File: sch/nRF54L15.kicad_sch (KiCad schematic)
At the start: 13 parts, among them U2 nPM1300-QEXX

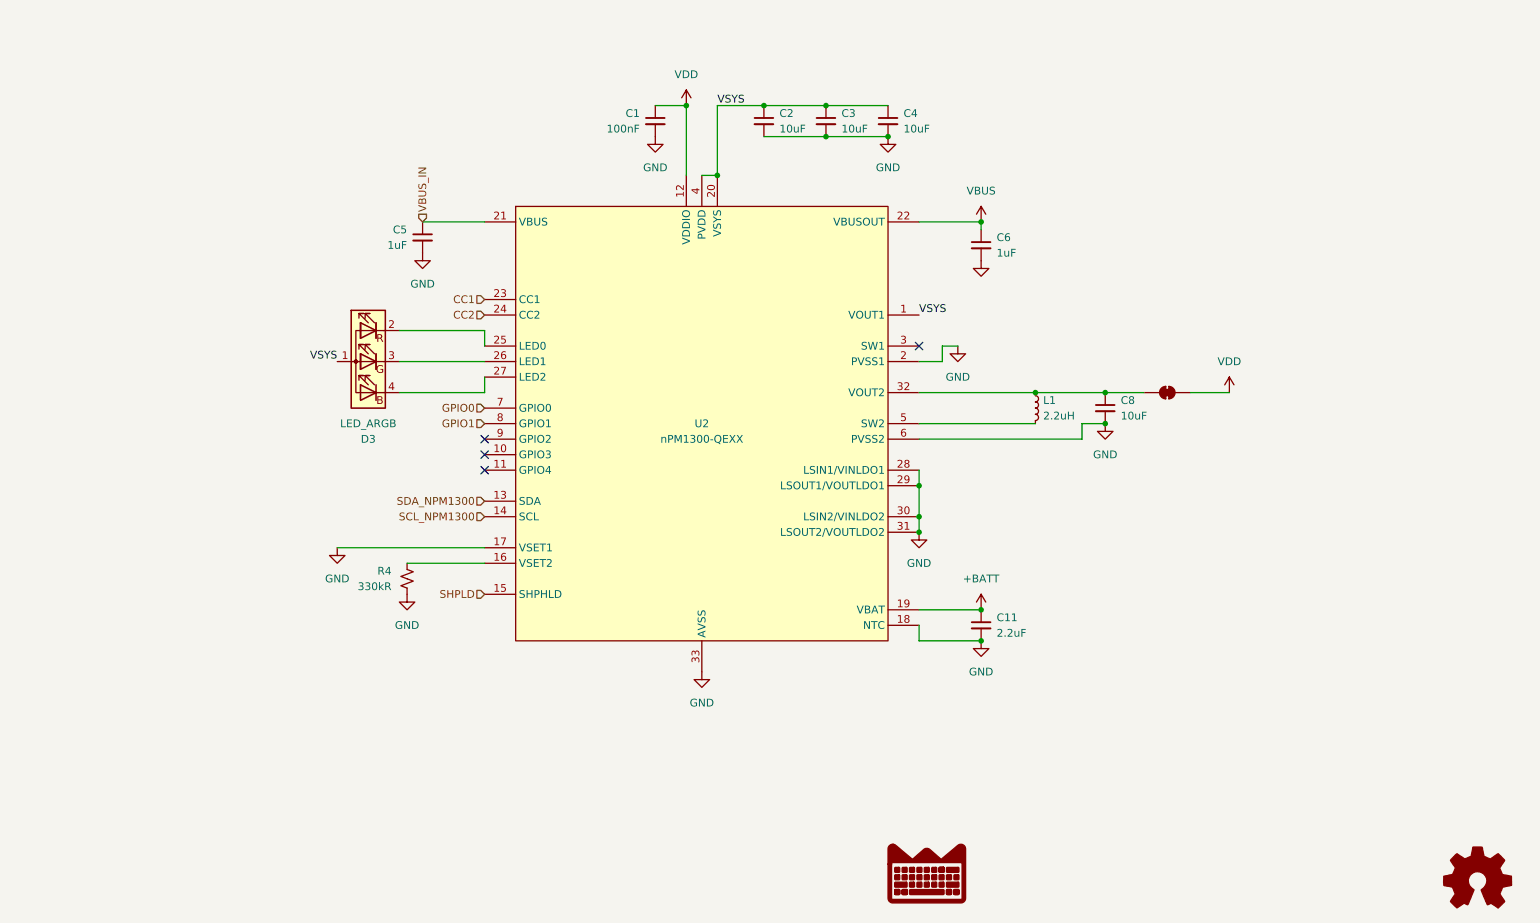
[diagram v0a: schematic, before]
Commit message: Updated 02/03/25
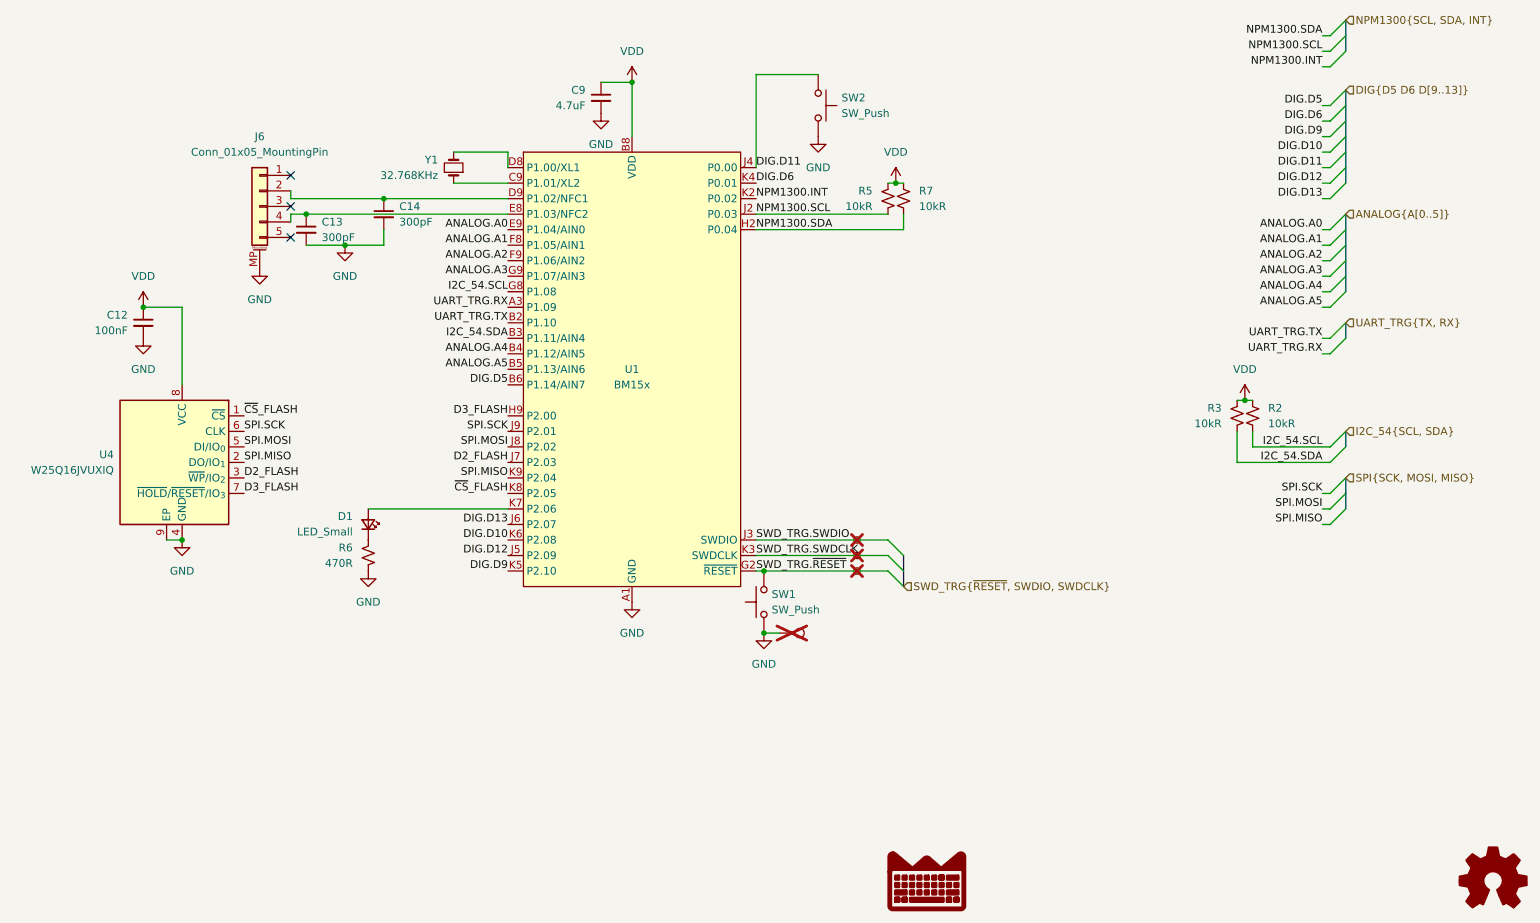
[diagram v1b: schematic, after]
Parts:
- removed C1: 100nF, Capacitor_SMD:C_0402_1005Metric, symbol Device:C_Small
- removed C11: 2.2uF, Capacitor_SMD:C_0603_1608Metric, symbol Device:C_Small
- removed C2, C3, C4, C8: 10uF, Capacitor_SMD:C_0603_1608Metric, symbol Device:C_Small
- removed C5, C6: 1uF, Capacitor_SMD:C_0603_1608Metric, symbol Device:C_Small
- removed D3: LED_ARGB, LED_SMD:LED_Wurth_150044M155260, symbol Device:LED_ARGB
- removed JP1: SolderJumper_2_Bridged, Jumper:SolderJumper-2_P1.3mm_Bridged_RoundedPad1.0x1.5mm, symbol Jumper:SolderJumper_2_Bridged
- removed L1: 2.2uH, Inductor_SMD:L_0603_1608Metric, symbol Device:L_Small
- removed R4: 330kR, Resistor_SMD:R_0402_1005Metric, symbol Device:R_Small_US
- removed U2: nPM1300-QEXX, Package_DFN_QFN:QFN-32-1EP_5x5mm_P0.5mm_EP3.6x3.6mm_ThermalVias, symbol nordic-lib-kicad-npm:nPM1300-QEXX
- added C12: 100nF, Capacitor_SMD:C_0402_1005Metric, symbol Device:C_Small
- added C13, C14: 300pF, Capacitor_SMD:C_0402_1005Metric, symbol Device:C_Small
- added C9: 4.7uF, Capacitor_SMD:C_0402_1005Metric, symbol Device:C_Small
- added D1: LED_Small, LED_SMD:LED_0603_1608Metric, symbol Device:LED_Small
- added J6: Conn_01x05_MountingPin, RoyalBlue-nRF54L15-Connector_FFC-FPC:CONN-SMD_5P-P0.50_HCTL_HC-FPC-05-09-5RLTAG, symbol Connector_Generic_MountingPin:Conn_01x05_MountingPin
- added R2, R3, R5, R7: 10kR, Resistor_SMD:R_0402_1005Metric, symbol Device:R_Small_US
- added R6: 470R, Resistor_SMD:R_0402_1005Metric, symbol Device:R_Small_US
- added SW1, SW2: SW_Push, Button_Switch_SMD:SW_Push_1P1T_NO_Vertical_Wuerth_434133025816, symbol Switch:SW_Push
- added TP1, TP2, TP3: TestPoint, TestPoint:TestPoint_Pad_D2.0mm, symbol Connector:TestPoint_Small
- added TP4: TestPoint, TestPoint:TestPoint_Pad_D2.0mm, symbol Connector:TestPoint
- added U1: BM15x, nordic-lib-kicad-nrf54-modules:BM15x-LGA-45_15.8x10mm, symbol nordic-lib-kicad-nrf54-modules:BM15x
- added U4: W25Q16JVUXIQ, Package_SON:Winbond_USON-8-1EP_3x2mm_P0.5mm_EP0.2x1.6mm, symbol Memory_Flash:W25Q32JVZP
- added Y1: 32.768KHz, Crystal:Crystal_SMD_3215-2Pin_3.2x1.5mm, symbol Device:Crystal_Small
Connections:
- net GND: now also C12.2, C13.2, C14.2, C9.2, J6.MP (MountPin), R6.2, SW1.1, SW2.2, TP4.1, U1.A1 (GND), U1.A9 (GND), U1.B1 (GND), U1.B7 (GND), U1.B9 (GND), U1.D1 (GND), U1.E1 (GND), U1.F1 (GND), U1.H8 (GND), U4.4 (GND), U4.9 (EP)
- net VDD: now also C12.1, C9.1, R2.1, R3.1, R5.1, R7.1, U1.B8 (VDD), U1.C8 (VDD), U4.8 (VCC)
- new net: D1.1 (K), R6.1
- new net: D1.2 (A), U1.K7 (P2.06)
- new net: U1.C9 (P1.01/XL2), Y1.1
- new net: U1.D8 (P1.00/XL1), Y1.2
- new net: C14.1, J6.2 (Pin_2), U1.D9 (P1.02/NFC1)
- new net: C13.1, J6.4 (Pin_4), U1.E8 (P1.03/NFC2)
- new net ANALOG.A0: U1.E9 (P1.04/AIN0)
- new net ANALOG.A1: U1.F8 (P1.05/AIN1)
- new net ANALOG.A2: U1.F9 (P1.06/AIN2)
- new net ANALOG.A3: U1.G9 (P1.07/AIN3)
- new net ANALOG.A4: U1.B4 (P1.12/AIN5)
- new net ANALOG.A5: U1.B5 (P1.13/AIN6)
- new net D2_FLASH: U1.J7 (P2.03), U4.3 (~{WP}/IO_{2})
- new net D3_FLASH: U1.H9 (P2.00), U4.7 (~{HOLD}/~{RESET}/IO_{3})
- new net DIG.D10: U1.K6 (P2.08)
- new net DIG.D11: SW2.1, U1.J4 (P0.00)
- new net DIG.D12: U1.J5 (P2.09)
- new net DIG.D13: U1.J6 (P2.07)
- new net DIG.D5: U1.B6 (P1.14/AIN7)
- new net DIG.D6: U1.K4 (P0.01)
- new net DIG.D9: U1.K5 (P2.10)
- new net I2C_54.SCL: R2.2, U1.G8 (P1.08)
- new net I2C_54.SDA: R3.2, U1.B3 (P1.11/AIN4)
- new net NPM1300.INT: U1.K2 (P0.02)
- new net NPM1300.SCL: R5.2, U1.J2 (P0.03)
- new net NPM1300.SDA: R7.2, U1.H2 (P0.04)
- new net SPI.MISO: U1.K9 (P2.04), U4.2 (DO/IO_{1})
- new net SPI.MOSI: U1.J8 (P2.02), U4.5 (DI/IO_{0})
- new net SPI.SCK: U1.J9 (P2.01), U4.6 (CLK)
- new net SWD_TRG.SWDCLK: TP3.1, U1.K3 (SWDCLK)
- new net SWD_TRG.SWDIO: TP1.1, U1.J3 (SWDIO)
- new net SWD_TRG.~{RESET}: SW1.2, TP2.1, U1.G2 (~{RESET})
- new net UART_TRG.RX: U1.A3 (P1.09)
- new net UART_TRG.TX: U1.B2 (P1.10)
- new net ~{CS}_FLASH: U1.K8 (P2.05), U4.1 (~{CS})
- no-connect marks 4 -> 3
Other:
- company: Lord's Boards -> (none)
- title: RoyalBlue54L -> (none)

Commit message: Renamed to RoyalBlue54L-Feather
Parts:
- J6: footprint RoyalBlue-nRF54L15-Connector_FFC-FPC:CONN-SMD_5P-P0.50_HCTL_HC-FPC-05-09-5RLTAG -> RoyalBlue54L-Feather-Connector_FFC-FPC:CONN-SMD_5P-P0.50_HCTL_HC-FPC-05-09-5RLTAG
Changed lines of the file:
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@@
 		)
 		(instances
-			(project "RoyalBlue-nRF54L15"
+			(project "RoyalBlue54L-Feather"
 				(path "/ba76ff89-c129-45ae-a3c9-97538370856c/b280f472-530c-47a8-bd61-35bd1befbf04"
 					(reference "#PWR045")
@@
 		)
 		(instances
-			(project "RoyalBlue-nRF54L15"
+			(project "RoyalBlue54L-Feather"
 				(path "/ba76ff89-c129-45ae-a3c9-97538370856c/b280f472-530c-47a8-bd61-35bd1befbf04"
 					(reference "D1")
@@
 		)
 		(instances
-			(project "RoyalBlue-nRF54L15"
+			(project "RoyalBlue54L-Feather"
 				(path "/ba76ff89-c129-45ae-a3c9-97538370856c/b280f472-530c-47a8-bd61-35bd1befbf04"
 					(reference "U4")
@@
 		)
 		(instances
-			(project "RoyalBlue-nRF54L15"
+			(project "RoyalBlue54L-Feather"
 				(path "/ba76ff89-c129-45ae-a3c9-97538370856c/b280f472-530c-47a8-bd61-35bd1befbf04"
 					(reference "R5")
@@
 		)
 		(instances
-			(project "RoyalBlue-nRF54L15"
+			(project "RoyalBlue54L-Feather"
 				(path "/ba76ff89-c129-45ae-a3c9-97538370856c/b280f472-530c-47a8-bd61-35bd1befbf04"
 					(reference "#PWR010")
@@
 		)
 		(instances
-			(project "RoyalBlue-nRF54L15"
+			(project "RoyalBlue54L-Feather"
 				(path "/ba76ff89-c129-45ae-a3c9-97538370856c/b280f472-530c-47a8-bd61-35bd1befbf04"
 					(reference "Y1")
@@
 		)
 		(instances
-			(project "RoyalBlue-nRF54L15"
+			(project "RoyalBlue54L-Feather"
 				(path "/ba76ff89-c129-45ae-a3c9-97538370856c/b280f472-530c-47a8-bd61-35bd1befbf04"
 					(reference "R3")
@@
 		)
 		(instances
-			(project "RoyalBlue-nRF54L15"
+			(project "RoyalBlue54L-Feather"
 				(path "/ba76ff89-c129-45ae-a3c9-97538370856c/b280f472-530c-47a8-bd61-35bd1befbf04"
 					(reference "U1")
@@
 		)
 		(instances
-			(project "RoyalBlue-nRF54L15"
+			(project "RoyalBlue54L-Feather"
 				(path "/ba76ff89-c129-45ae-a3c9-97538370856c/b280f472-530c-47a8-bd61-35bd1befbf04"
 					(reference "#SYM7")
@@
 			)
 		)
-		(property "Footprint" "RoyalBlue-nRF54L15-Connector_FFC-FPC:CONN-SMD_5P-P0.50_HCTL_HC-FPC-05-09-5RLTAG"
+		(property "Footprint" "RoyalBlue54L-Feather-Connector_FFC-FPC:CONN-SMD_5P-P0.50_HCTL_HC-FPC-05-09-5RLTAG"
 			(at 76.2 63.5 0)
 			(effects
@@
 		)
 		(instances
-			(project "RoyalBlue-nRF54L15"
+			(project "RoyalBlue54L-Feather"
 				(path "/ba76ff89-c129-45ae-a3c9-97538370856c/b280f472-530c-47a8-bd61-35bd1befbf04"
 					(reference "J6")
@@
 		)
 		(instances
-			(project "RoyalBlue-nRF54L15"
+			(project "RoyalBlue54L-Feather"
 				(path "/ba76ff89-c129-45ae-a3c9-97538370856c/b280f472-530c-47a8-bd61-35bd1befbf04"
 					(reference "R7")
@@
 		)
 		(instances
-			(project "RoyalBlue-nRF54L15"
+			(project "RoyalBlue54L-Feather"
 				(path "/ba76ff89-c129-45ae-a3c9-97538370856c/b280f472-530c-47a8-bd61-35bd1befbf04"
 					(reference "#PWR043")
@@
 		)
 		(instances
-			(project "RoyalBlue-nRF54L15"
+			(project "RoyalBlue54L-Feather"
 				(path "/ba76ff89-c129-45ae-a3c9-97538370856c/b280f472-530c-47a8-bd61-35bd1befbf04"
 					(reference "#PWR011")
@@
 		)
 		(instances
-			(project "RoyalBlue-nRF54L15"
+			(project "RoyalBlue54L-Feather"
 				(path "/ba76ff89-c129-45ae-a3c9-97538370856c/b280f472-530c-47a8-bd61-35bd1befbf04"
 					(reference "#PWR014")
@@
 		)
 		(instances
-			(project "RoyalBlue-nRF54L15"
+			(project "RoyalBlue54L-Feather"
 				(path "/ba76ff89-c129-45ae-a3c9-97538370856c/b280f472-530c-47a8-bd61-35bd1befbf04"
 					(reference "C13")
@@
 		)
 		(instances
-			(project "RoyalBlue-nRF54L15"
+			(project "RoyalBlue54L-Feather"
 				(path "/ba76ff89-c129-45ae-a3c9-97538370856c/b280f472-530c-47a8-bd61-35bd1befbf04"
 					(reference "R2")
@@
 		)
 		(instances
-			(project "RoyalBlue-nRF54L15"
+			(project "RoyalBlue54L-Feather"
 				(path "/ba76ff89-c129-45ae-a3c9-97538370856c/b280f472-530c-47a8-bd61-35bd1befbf04"
 					(reference "SW2")
@@
 		)
 		(instances
-			(project "RoyalBlue-nRF54L15"
+			(project "RoyalBlue54L-Feather"
 				(path "/ba76ff89-c129-45ae-a3c9-97538370856c/b280f472-530c-47a8-bd61-35bd1befbf04"
 					(reference "#PWR039")
@@
 		)
 		(instances
-			(project "RoyalBlue-nRF54L15"
+			(project "RoyalBlue54L-Feather"
 				(path "/ba76ff89-c129-45ae-a3c9-97538370856c/b280f472-530c-47a8-bd61-35bd1befbf04"
 					(reference "#PWR038")
@@
 		)
 		(instances
-			(project "RoyalBlue-nRF54L15"
+			(project "RoyalBlue54L-Feather"
 				(path "/ba76ff89-c129-45ae-a3c9-97538370856c/b280f472-530c-47a8-bd61-35bd1befbf04"
 					(reference "TP1")
@@
 		)
 		(instances
-			(project "RoyalBlue-nRF54L15"
+			(project "RoyalBlue54L-Feather"
 				(path "/ba76ff89-c129-45ae-a3c9-97538370856c/b280f472-530c-47a8-bd61-35bd1befbf04"
 					(reference "#PWR052")
@@
 		)
 		(instances
-			(project "RoyalBlue-nRF54L15"
+			(project "RoyalBlue54L-Feather"
 				(path "/ba76ff89-c129-45ae-a3c9-97538370856c/b280f472-530c-47a8-bd61-35bd1befbf04"
 					(reference "TP2")
@@
 		)
 		(instances
-			(project "RoyalBlue-nRF54L15"
+			(project "RoyalBlue54L-Feather"
 				(path "/ba76ff89-c129-45ae-a3c9-97538370856c/b280f472-530c-47a8-bd61-35bd1befbf04"
 					(reference "C9")
@@
 		)
 		(instances
-			(project "RoyalBlue-nRF54L15"
+			(project "RoyalBlue54L-Feather"
 				(path "/ba76ff89-c129-45ae-a3c9-97538370856c/b280f472-530c-47a8-bd61-35bd1befbf04"
 					(reference "#PWR037")
@@
 		)
 		(instances
-			(project "RoyalBlue-nRF54L15"
+			(project "RoyalBlue54L-Feather"
 				(path "/ba76ff89-c129-45ae-a3c9-97538370856c/b280f472-530c-47a8-bd61-35bd1befbf04"
 					(reference "#PWR050")
@@
 		)
 		(instances
-			(project "RoyalBlue-nRF54L15"
+			(project "RoyalBlue54L-Feather"
 				(path "/ba76ff89-c129-45ae-a3c9-97538370856c/b280f472-530c-47a8-bd61-35bd1befbf04"
 					(reference "C12")
@@
 		)
 		(instances
-			(project "RoyalBlue-nRF54L15"
+			(project "RoyalBlue54L-Feather"
 				(path "/ba76ff89-c129-45ae-a3c9-97538370856c/b280f472-530c-47a8-bd61-35bd1befbf04"
 					(reference "SW1")
@@
 		)
 		(instances
-			(project "RoyalBlue-nRF54L15"
+			(project "RoyalBlue54L-Feather"
 				(path "/ba76ff89-c129-45ae-a3c9-97538370856c/b280f472-530c-47a8-bd61-35bd1befbf04"
 					(reference "#PWR051")
@@
 		)
 		(instances
-			(project "RoyalBlue-nRF54L15"
+			(project "RoyalBlue54L-Feather"
 				(path "/ba76ff89-c129-45ae-a3c9-97538370856c/b280f472-530c-47a8-bd61-35bd1befbf04"
 					(reference "TP4")
@@
 		)
 		(instances
-			(project "RoyalBlue-nRF54L15"
+			(project "RoyalBlue54L-Feather"
 				(path "/ba76ff89-c129-45ae-a3c9-97538370856c/b280f472-530c-47a8-bd61-35bd1befbf04"
 					(reference "TP3")
@@
 		)
 		(instances
-			(project "RoyalBlue-nRF54L15"
+			(project "RoyalBlue54L-Feather"
 				(path "/ba76ff89-c129-45ae-a3c9-97538370856c/b280f472-530c-47a8-bd61-35bd1befbf04"
 					(reference "#SYM8")
@@
 		)
 		(instances
-			(project "RoyalBlue-nRF54L15"
+			(project "RoyalBlue54L-Feather"
 				(path "/ba76ff89-c129-45ae-a3c9-97538370856c/b280f472-530c-47a8-bd61-35bd1befbf04"
 					(reference "R6")
@@
 		)
 		(instances
-			(project "RoyalBlue-nRF54L15"
+			(project "RoyalBlue54L-Feather"
 				(path "/ba76ff89-c129-45ae-a3c9-97538370856c/b280f472-530c-47a8-bd61-35bd1befbf04"
 					(reference "#PWR026")
@@
 		)
 		(instances
-			(project "RoyalBlue-nRF54L15"
+			(project "RoyalBlue54L-Feather"
 				(path "/ba76ff89-c129-45ae-a3c9-97538370856c/b280f472-530c-47a8-bd61-35bd1befbf04"
 					(reference "C14")
@@
 		)
 		(instances
-			(project "RoyalBlue-nRF54L15"
+			(project "RoyalBlue54L-Feather"
 				(path "/ba76ff89-c129-45ae-a3c9-97538370856c/b280f472-530c-47a8-bd61-35bd1befbf04"
 					(reference "#PWR046")
